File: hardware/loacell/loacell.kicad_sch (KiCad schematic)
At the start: 7 parts, among them J1 Conn_01x04_Male, U1 INA128, U2 D1_mini_battery_shield, U3 ESP32-DEVKIT-V1

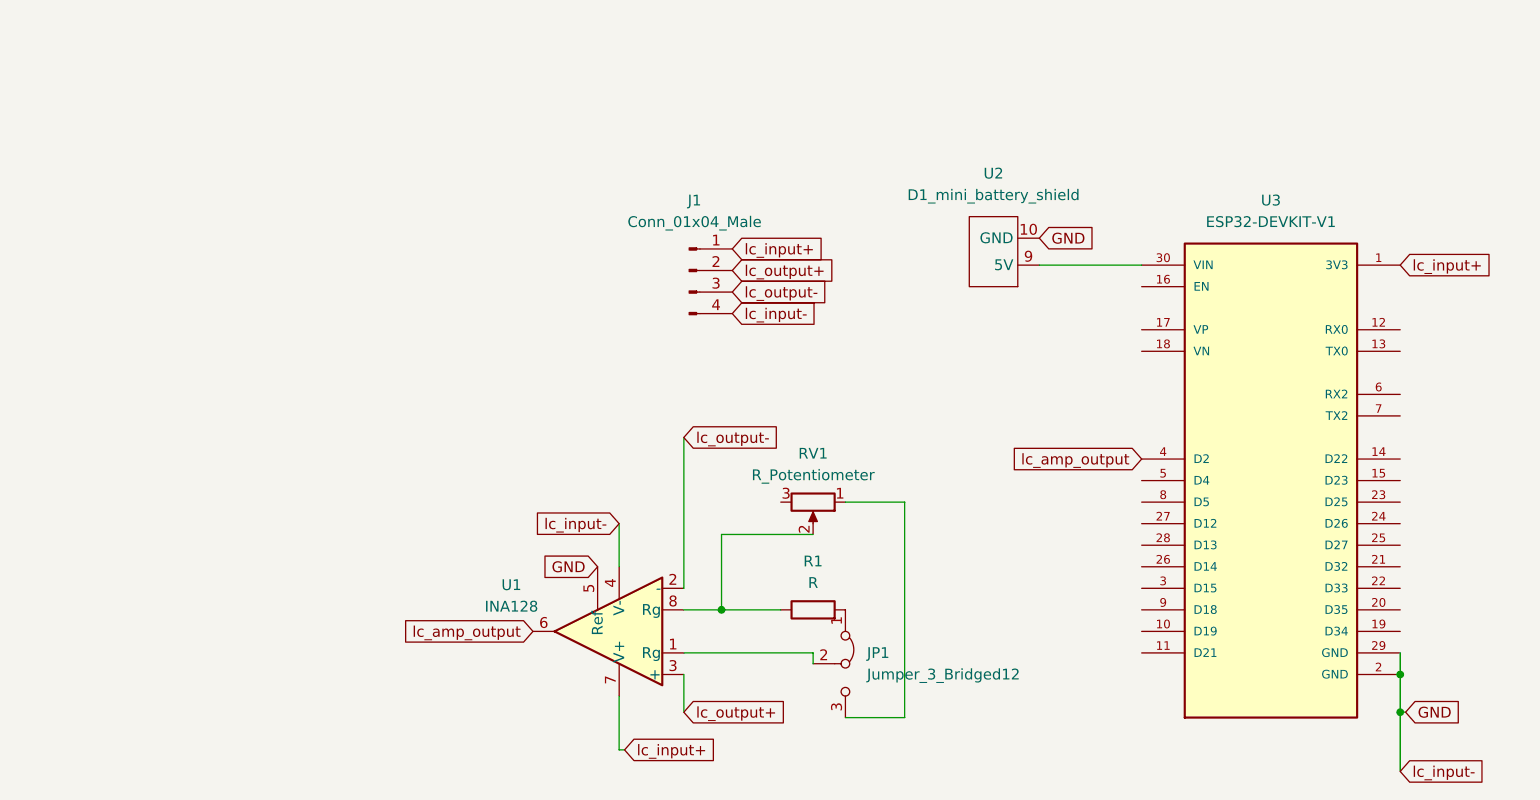
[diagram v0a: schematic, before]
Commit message: init
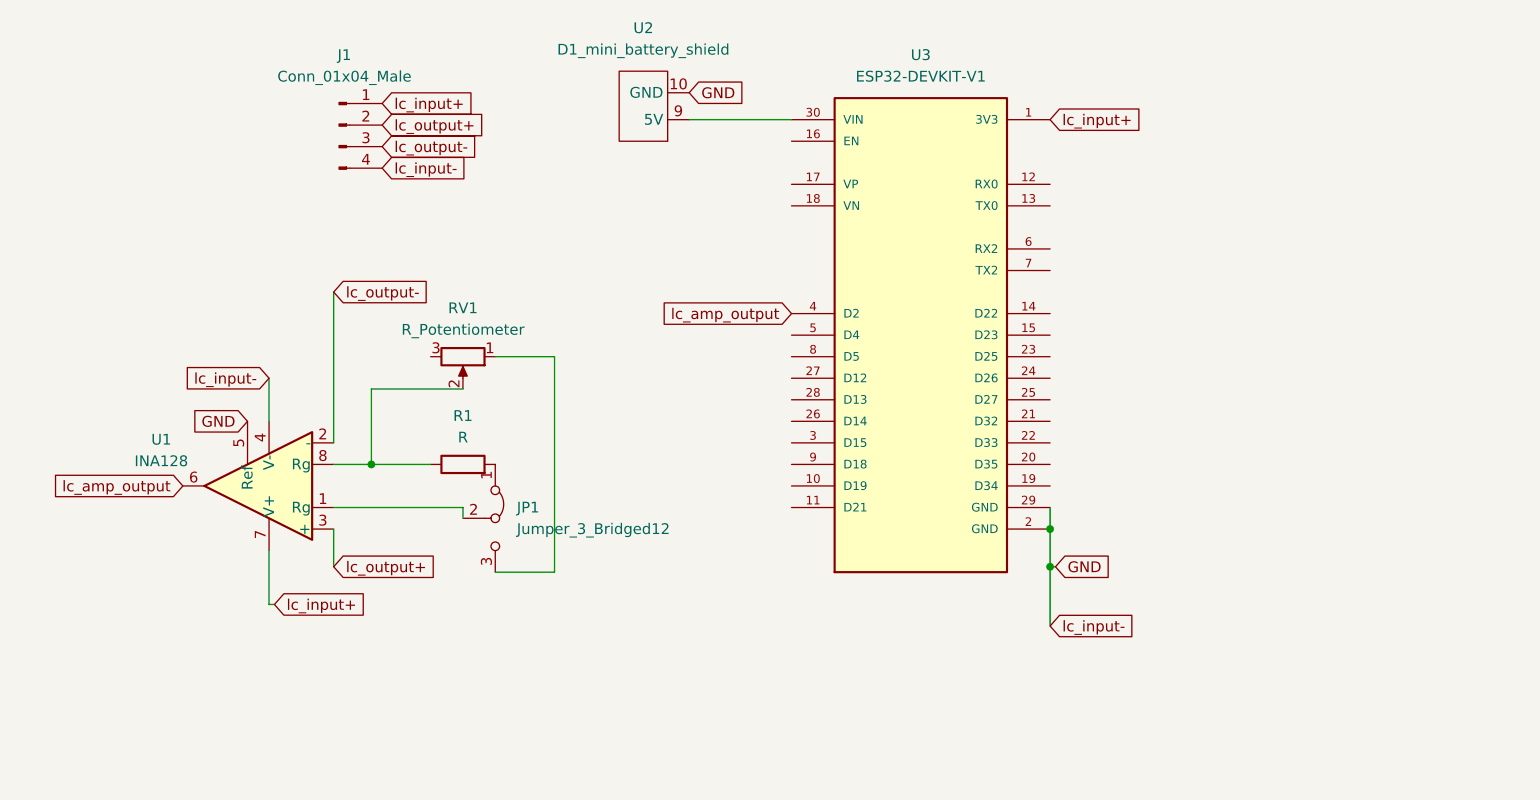
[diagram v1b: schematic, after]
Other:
- title: (none) -> LOADCELL
- moved on the sheet: J1, JP1, R1, RV1, U1, U2, U3
